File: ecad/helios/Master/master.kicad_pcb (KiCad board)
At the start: 2 copper layers, 100 x 100 mm, 146 parts, among them J1 MCV 1,5/ 3-G-3,5, J10 MiniFit JR 5556 08A2, J11 MCV 1,5/ 2-G-3,5, J12 MiniFit JR 5556 08A2, J13 M20-8760342, J2 MCV 1,5/ 2-G-3,5, J3 MCV 1,5/ 2-G-3,5, J4 MCV 1,5/ 2-G-3,5, J5 MCV 1,5/ 2-G-3,5, J6 MiniFit JR 5556 08A2, J7 MCV 1,5/ 2-G-3,5, J8 MiniFit JR 5556 08A2, J9 MCV 1,5/ 2-G-3,5, Q1 IRF9Z34NPbF, Q2 BSS84P, Q3 IRF9Z34NPbF, Q4 BSS84P, Q5 IRF9Z34NPbF, Q6 BSS84P, Q7 IRF9Z34NPbF, Q8 BSS84P, SW1 1825910-6, U1 NCP1117-5.0_SOT223, U10 ISO7320FC, U11 UA9638, U12 LM2842Y, U13 LP3985IM5-5.0/NOPB, U14 TPS1H100AQPWPRQ1, U15 ISO7320FC, U16 UA9638, U17 LM2842Y, U18 LP3985IM5-5.0/NOPB, U19 TPS1H100AQPWPRQ1, U2 MCP2561-E/SN, U20 ISO7320FC, U21 UA9638, U22 LM2842Y, U23 LP3985IM5-5.0/NOPB, U3 ATMEGA16M1-AU, U4 TPS1H100AQPWPRQ1, U5 ISO7320FC, U6 UA9638, U7 LM2842Y, U8 LP3985IM5-5.0/NOPB, U9 TPS1H100AQPWPRQ1, Y1 16MHz

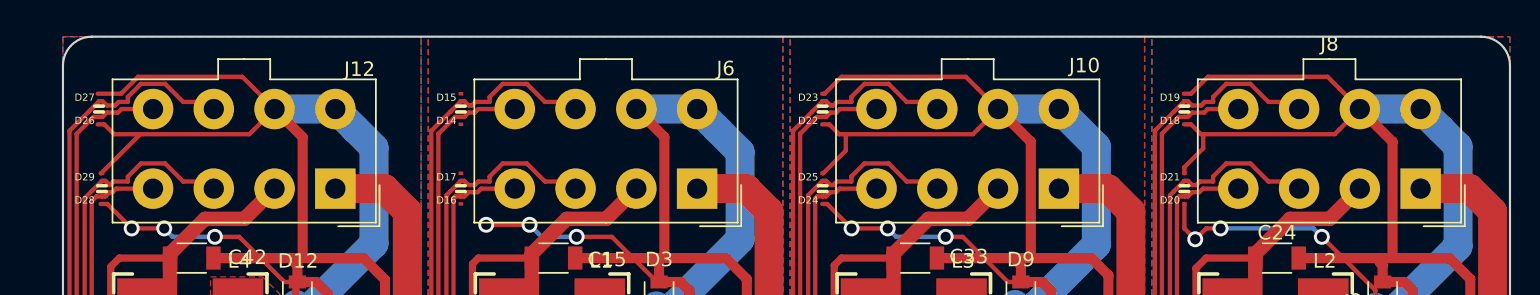
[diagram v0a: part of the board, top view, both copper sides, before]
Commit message: wip
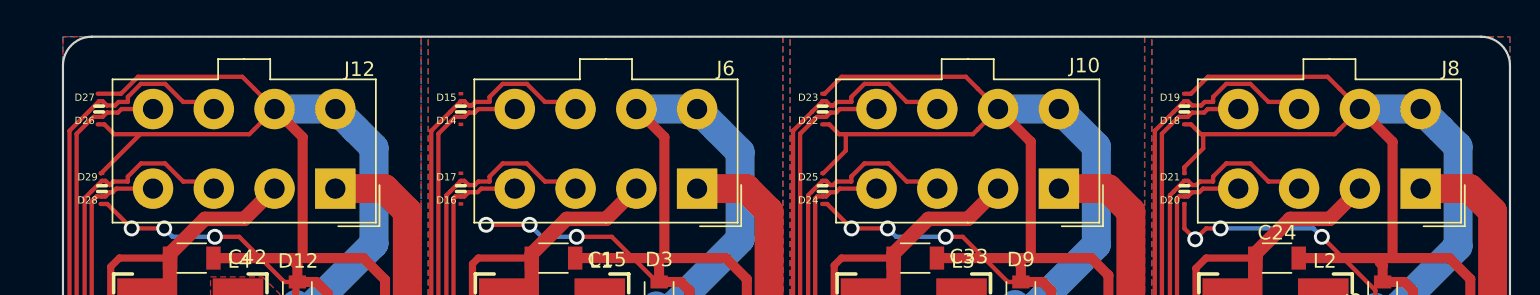
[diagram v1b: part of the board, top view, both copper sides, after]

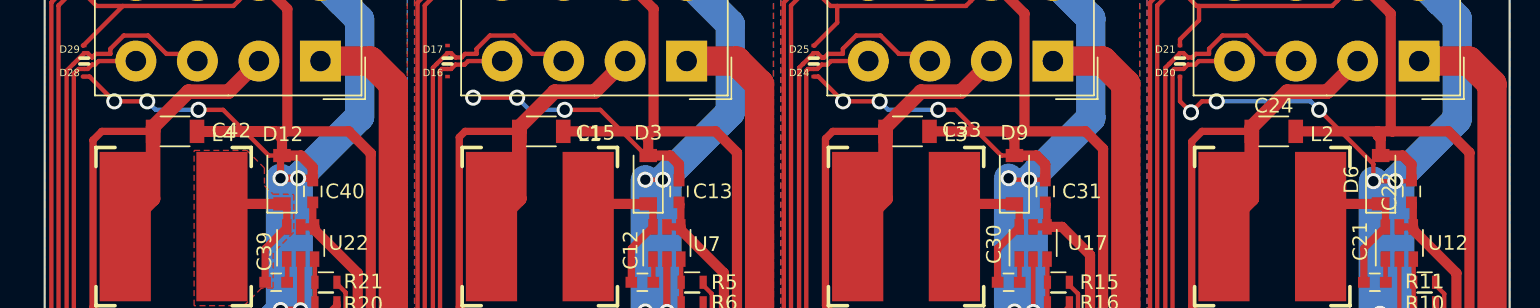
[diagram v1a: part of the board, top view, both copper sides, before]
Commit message: wip
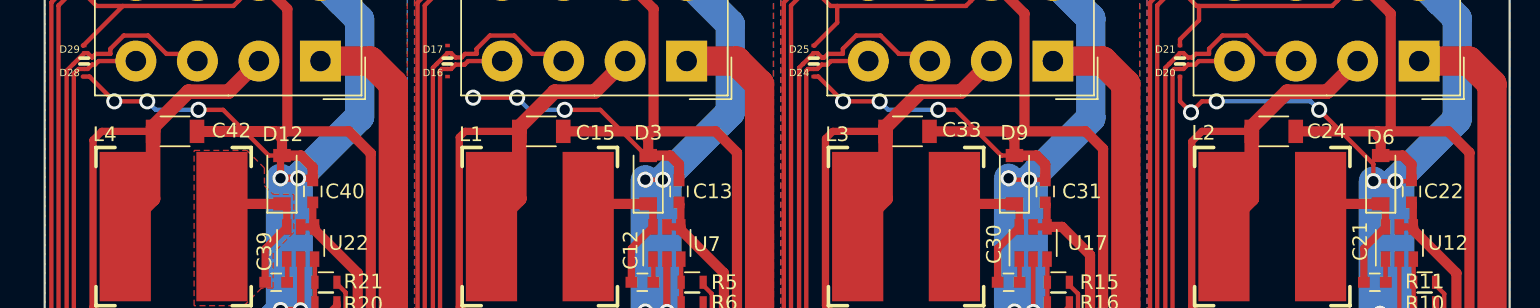
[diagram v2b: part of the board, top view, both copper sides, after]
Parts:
- C13, C22, C31, C40: value 1uF -> 1uF, 50V
- C17, C26, C35, C44: value 0.01uF -> 10nF, 50V
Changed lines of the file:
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@@
     (pad_to_mask_clearance 0.08)
     (aux_axis_origin 102.5 128.7)
-    (grid_origin 100 150)
+    (grid_origin 102.5 128.7)
     (visible_elements FFFFFF7F)
     (pcbplotparams
@@
       (viasonmask false)
       (mode 1)
-      (useauxorigin false)
+      (useauxorigin true)
       (hpglpennumber 1)
       (hpglpenspeed 20)
@@
       (effects (font (size 1 1) (thickness 0.15)))
     )
-    (fp_text value 1uF (at 0 1.5 90) (layer F.Fab)
+    (fp_text value "1uF, 50V" (at 0 1.5 90) (layer F.Fab)
       (effects (font (size 1 1) (thickness 0.15)))
     )
@@
       (effects (font (size 1 1) (thickness 0.15)))
     )
-    (fp_text value 0.01uF (at 0 1.5 270) (layer F.Fab)
+    (fp_text value "10nF, 50V" (at 0 1.5 270) (layer F.Fab)
       (effects (font (size 1 1) (thickness 0.15)))
     )
@@
     (tags "capacitor 0603")
     (attr smd)
-    (fp_text reference C22 (at 0 -1.5 90) (layer F.SilkS)
+    (fp_text reference C22 (at 0 2.2 180) (layer F.SilkS)
       (effects (font (size 1 1) (thickness 0.15)))
     )
-    (fp_text value 1uF (at 0 1.5 90) (layer F.Fab)
+    (fp_text value "1uF, 50V" (at 0 1.5 90) (layer F.Fab)
       (effects (font (size 1 1) (thickness 0.15)))
     )
@@
     (tags "capacitor 1206")
     (attr smd)
-    (fp_text reference C24 (at 0 -1.75) (layer F.SilkS)
+    (fp_text reference C24 (at 3.6 0) (layer F.SilkS)
       (effects (font (size 1 1) (thickness 0.15)))
     )
@@
       (effects (font (size 1 1) (thickness 0.15)))
     )
-    (fp_text value 0.01uF (at 0 1.5 270) (layer F.Fab)
+    (fp_text value "10nF, 50V" (at 0 1.5 270) (layer F.Fab)
       (effects (font (size 1 1) (thickness 0.15)))
     )
@@
       (effects (font (size 1 1) (thickness 0.15)))
     )
-    (fp_text value 1uF (at 0 1.5 90) (layer F.Fab)
+    (fp_text value "1uF, 50V" (at 0 1.5 90) (layer F.Fab)
       (effects (font (size 1 1) (thickness 0.15)))
     )
@@
       (effects (font (size 1 1) (thickness 0.15)))
     )
-    (fp_text value 0.01uF (at 0 1.5 270) (layer F.Fab)
+    (fp_text value "10nF, 50V" (at 0 1.5 270) (layer F.Fab)
       (effects (font (size 1 1) (thickness 0.15)))
     )
@@
       (effects (font (size 1 1) (thickness 0.15)))
     )
-    (fp_text value 1uF (at 0 1.5 90) (layer F.Fab)
+    (fp_text value "1uF, 50V" (at 0 1.5 90) (layer F.Fab)
       (effects (font (size 1 1) (thickness 0.15)))
     )
@@
       (effects (font (size 1 1) (thickness 0.15)))
     )
-    (fp_text value 0.01uF (at 0 1.5 270) (layer F.Fab)
+    (fp_text value "10nF, 50V" (at 0 1.5 270) (layer F.Fab)
       (effects (font (size 1 1) (thickness 0.15)))
     )
@@
     (tags SOD-123)
     (attr smd)
-    (fp_text reference D6 (at 0 -2 90) (layer F.SilkS)
+    (fp_text reference D6 (at 2.9 0 180) (layer F.SilkS)
       (effects (font (size 1 1) (thickness 0.15)))
     )
@@
     (at 133.8 71.8 180)
     (attr smd)
-    (fp_text reference L1 (at -3.4 6.3 180) (layer F.SilkS)
+    (fp_text reference L1 (at 4.7 6.3 180) (layer F.SilkS)
       (effects (font (size 1 1) (thickness 0.15)))
     )
@@
     (at 108.8 71.8 180)
     (attr smd)
-    (fp_text reference L4 (at -3.4 6.3 180) (layer F.SilkS)
+    (fp_text reference L4 (at 4.7 6.3 180) (layer F.SilkS)
       (effects (font (size 1 1) (thickness 0.15)))
     )
@@
     (at 158.8 71.8 180)
     (attr smd)
-    (fp_text reference L3 (at -3.4 6.3 180) (layer F.SilkS)
+    (fp_text reference L3 (at 4.7 6.3 180) (layer F.SilkS)
       (effects (font (size 1 1) (thickness 0.15)))
     )
@@
     (at 183.8 71.8 180)
     (attr smd)
-    (fp_text reference L2 (at -3.4 6.3 180) (layer F.SilkS)
+    (fp_text reference L2 (at 4.7 6.4 180) (layer F.SilkS)
       (effects (font (size 1 1) (thickness 0.15)))
     )
